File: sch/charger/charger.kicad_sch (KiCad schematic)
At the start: 90 parts, among them CON1 Conn_01x03, J1 0R, J1 Conn_01x02, Q1 CM4N60F, Q11 MMBT3904, Q12 MMBT3906, Q2 MMBT5551LT, Q5 4953, Q6 MMBT3904, U1 A4953_LJ, U1 LTV-817, U2 L78L05, U2 TL431DBZ

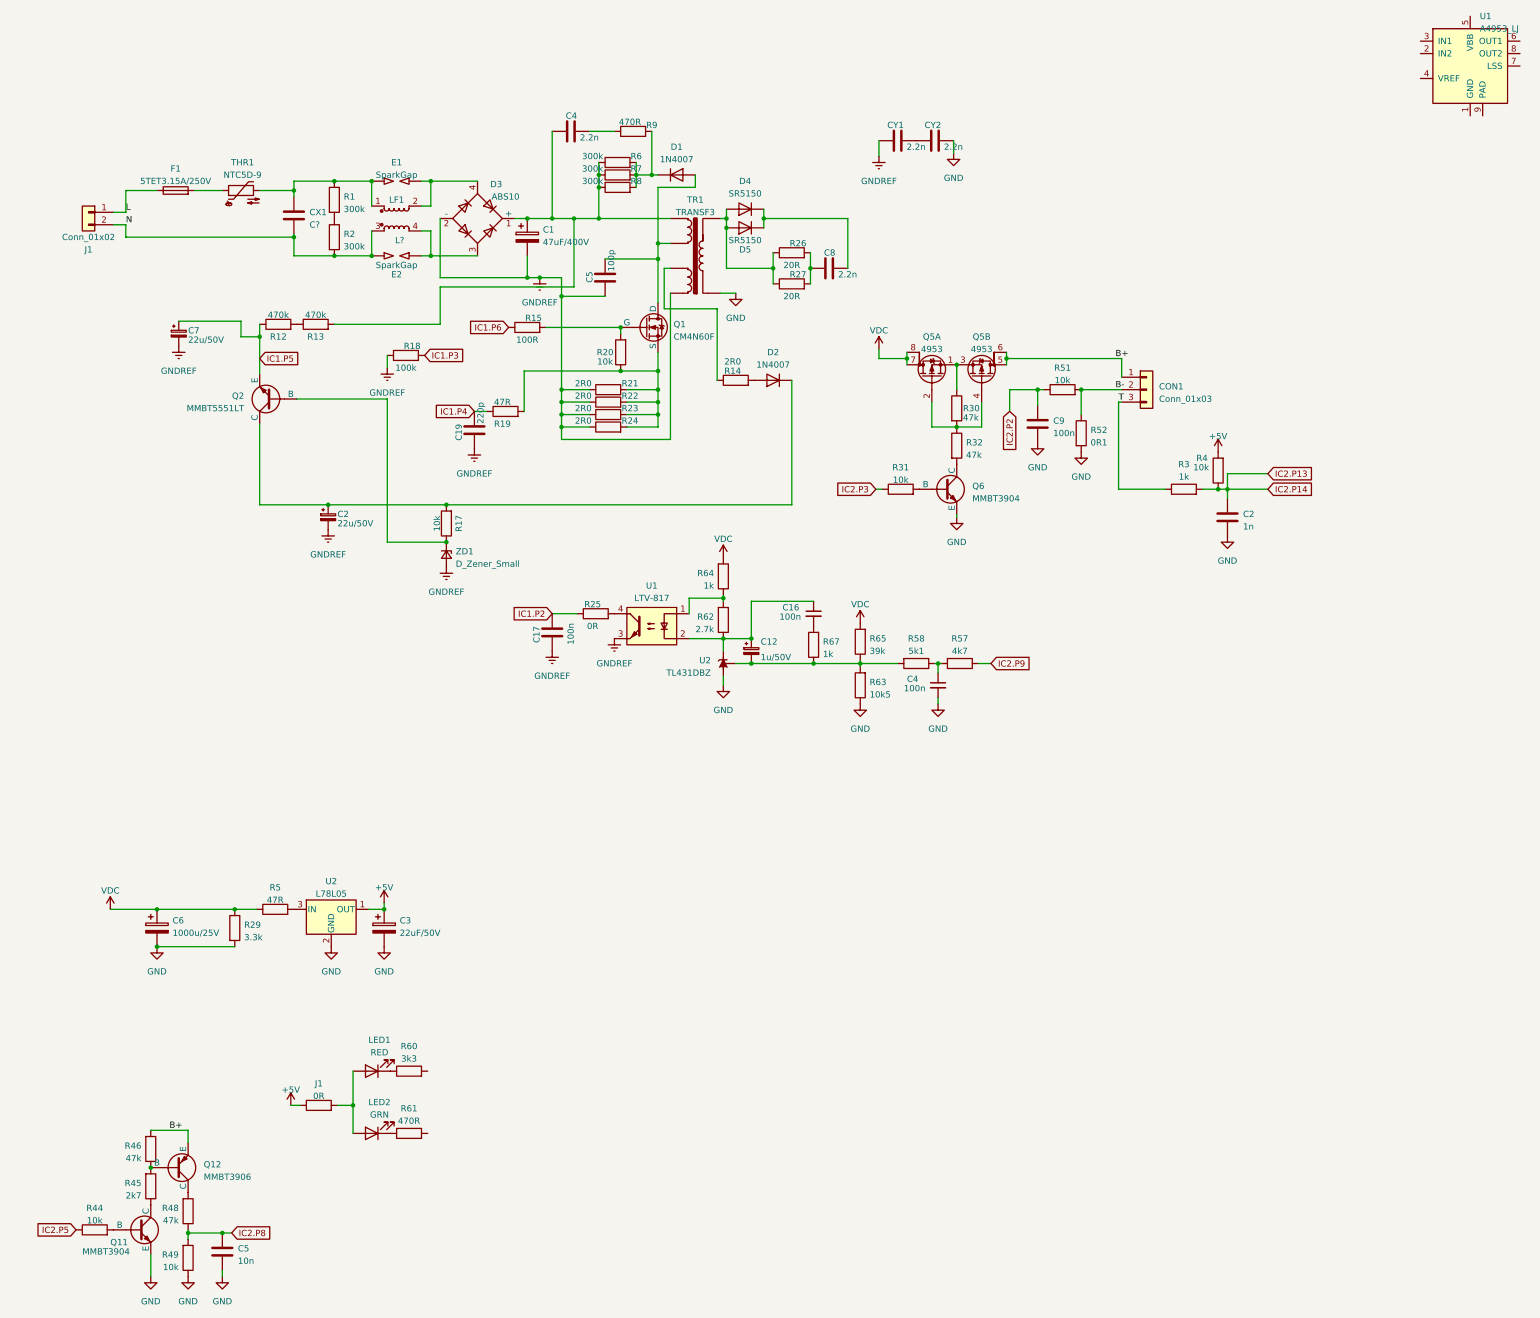
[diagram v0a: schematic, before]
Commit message: Cleanup schematic
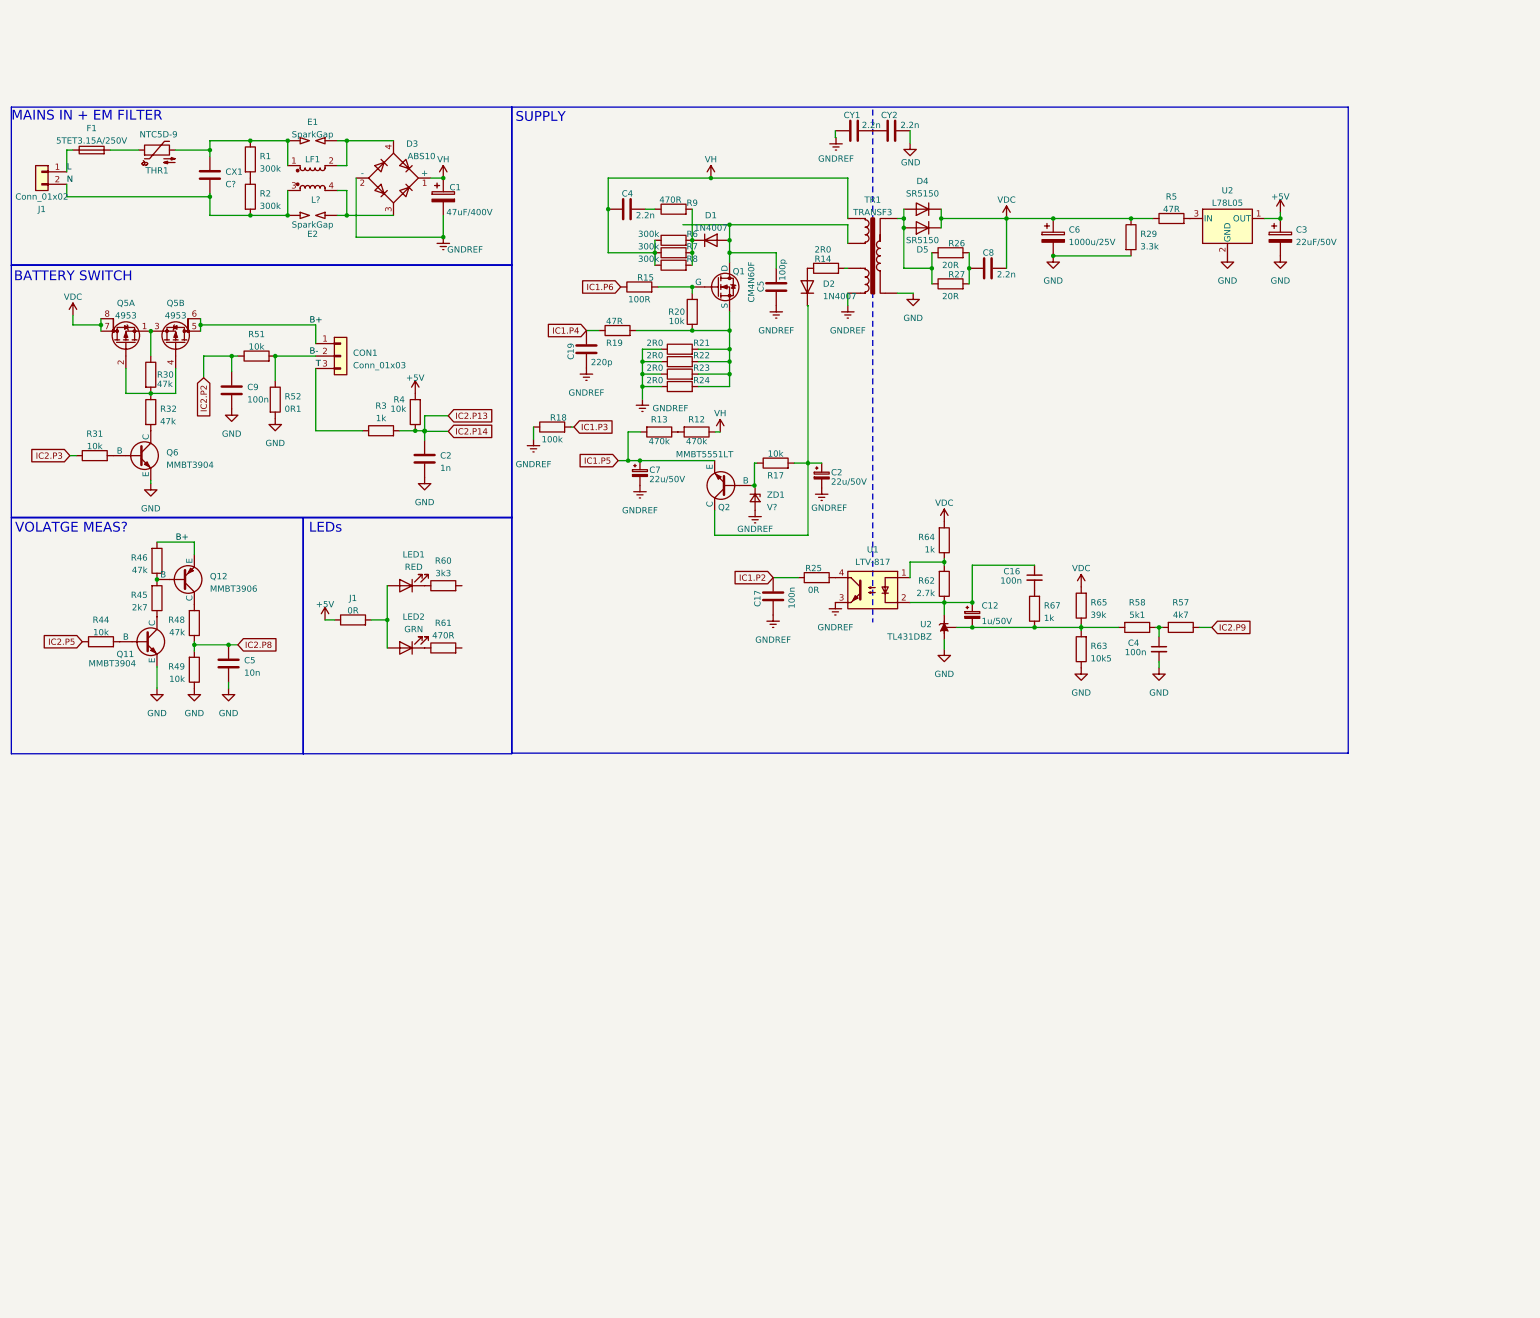
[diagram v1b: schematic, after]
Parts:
- removed U1: A4953_LJ, Package_SO:SOIC-8-1EP_3.9x4.9mm_P1.27mm_EP2.41x3.3mm, symbol Driver_Motor:A4953_LJ
- ZD1: value D_Zener_Small -> V?
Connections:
- net IC1.P5: now also R13.2; no longer R12.1
- net VDC: now also C8.2, D4.1 (K), D5.1 (K)
- net VDD: now reaches C1.1, C4.1, D3.1 (+), R6.1, R7.1, R8.1, TR1.6
- net VDD: now also R12.1; no longer R13.2
- net at R14.1: now also D2.2 (A); no longer TR1.4
- net at R14.2: now also TR1.4; no longer D2.2 (A)
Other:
- note added: "BATTERY SWITCH"
- note added: "LEDs"
- note added: "MAINS IN + EM FILTER"
- note added: "SUPPLY"
- note added: "VOLATGE MEAS?"
- moved on the sheet: C1, C12, C16, C17, C19, C2, C3, C4, C5, C6, C7, C8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
